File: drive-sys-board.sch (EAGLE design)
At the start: 33 parts

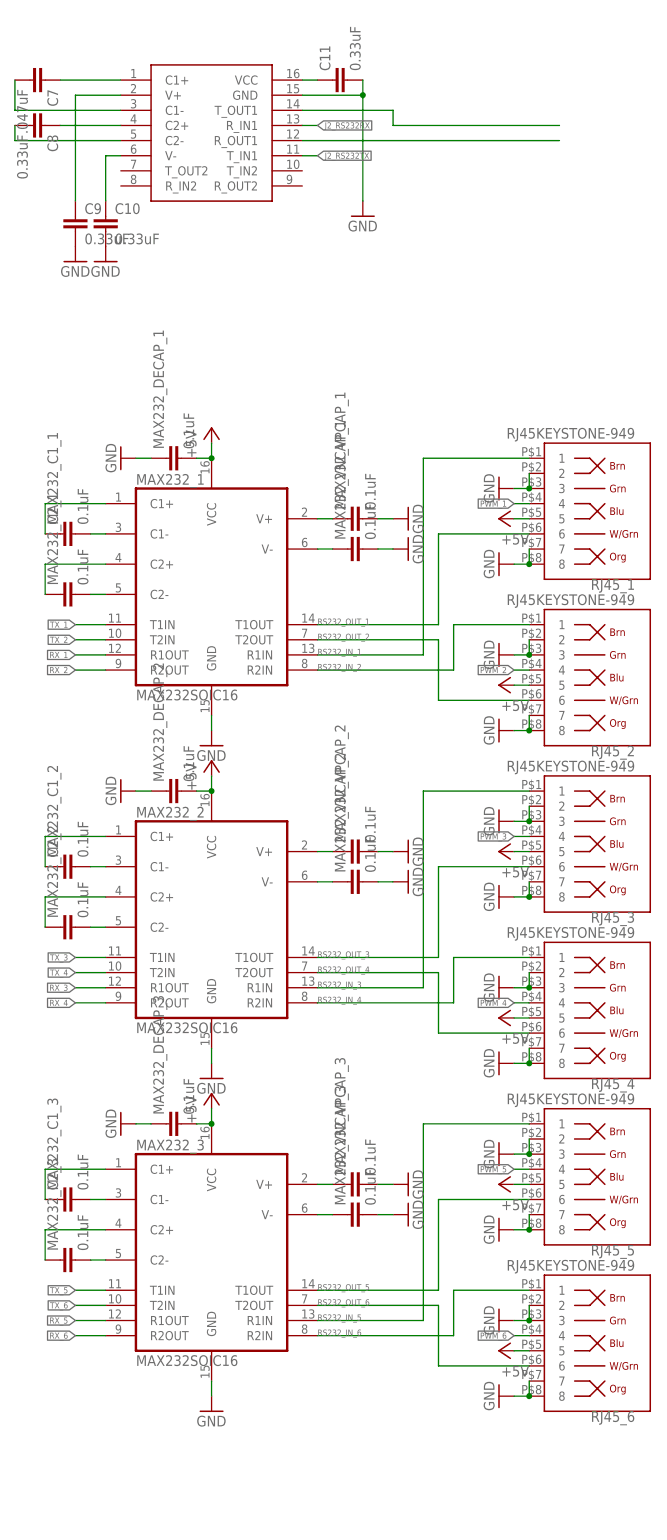
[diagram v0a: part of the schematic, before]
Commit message: final rs232 version
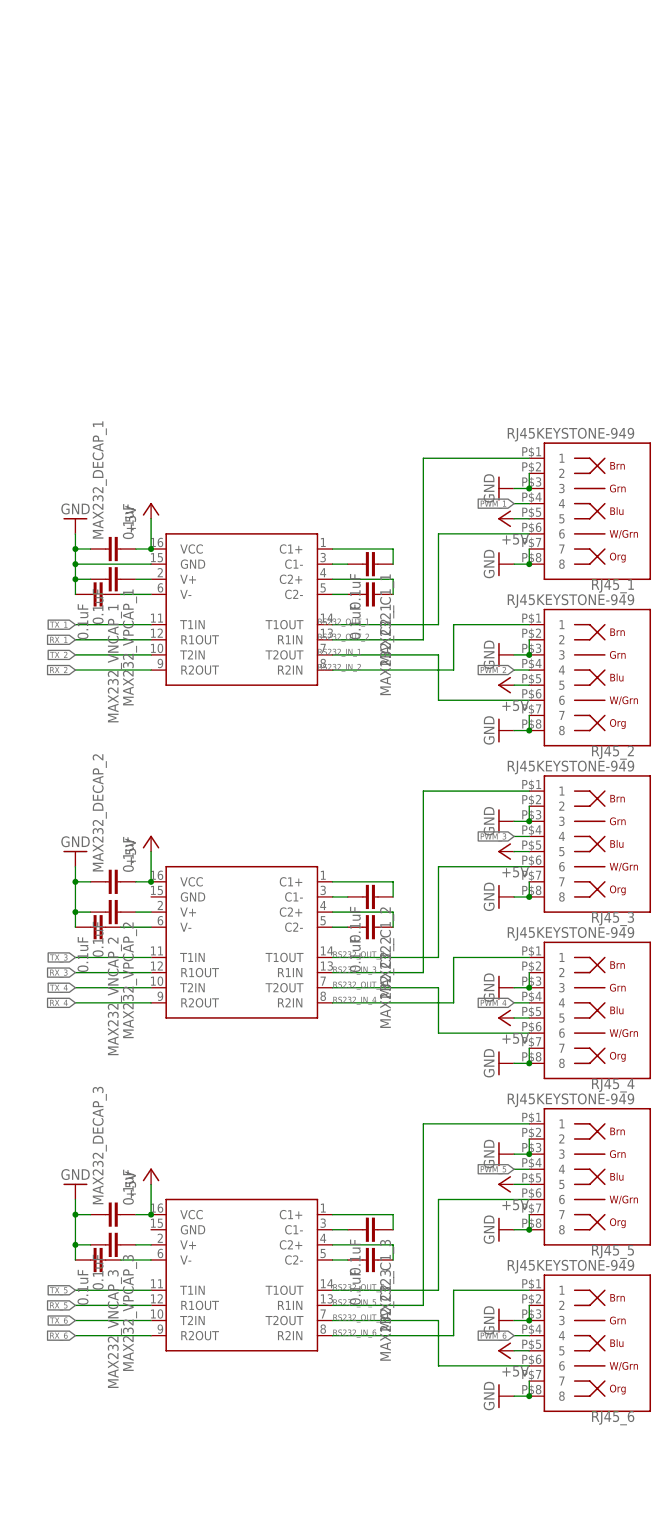
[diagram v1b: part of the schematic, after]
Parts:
- removed C10, C11, C8, C9: 0.33uF, SparkFun-Capacitors:CAP1206
- removed C7: .047uF, SparkFun-Capacitors:CAP1206
- removed MAX232: MAX3232, MRDT-LIB2014:MAX3232
- MAX232_1, MAX232_2, MAX232_3: value MAX232SOIC16 -> MAX3232SO16; device SparkFun-DigitalIC:MAX232SOIC16 -> MRDT-Digital-ICs:MAX3232SO16
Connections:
- removed net J2_RS232RX: MAX232.R_IN1
- removed net J2_RS232TX: MAX232.T_IN1
- removed net N$15: C7.2, MAX232.C1-
- removed net N$16: C7.1, MAX232.C1+
- removed net N$17: C8.1, MAX232.C2+
- removed net N$18: C8.2, MAX232.C2-
- removed net N$19: C10.1, MAX232.V-
- removed net N$20: C9.1, MAX232.V+
- removed net R_OUT1: MAX232.R_OUT1
- removed net T_OUT1: MAX232.T_OUT1
- removed net VCC1: C11.1, MAX232.VCC
- net GND: no longer C10.2, C11.2, C9.2, MAX232.GND, MAX232_2.GND, MAX232_3.GND
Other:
- moved on the sheet: MAX232_C1_1, MAX232_C1_2, MAX232_C1_3, MAX232_C2_1, MAX232_C2_2, MAX232_C2_3, MAX232_DECAP_1, MAX232_DECAP_2, MAX232_DECAP_3, MAX232_VNCAP_1, MAX232_VNCAP_2, MAX232_VNCAP_3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
